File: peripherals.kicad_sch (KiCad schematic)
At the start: 36 parts, among them IC1 MIC5350-SGYMT-TR, J1 Conn_02x06_Counter_Clockwise, J2 USB_C_Receptacle_USB2.0_14P, J3 Conn_01x07, J4 Conn_01x06, J5 Conn_02x08_Odd_Even, U1 EM008LX, U2 EM008LX, U3 EM008LX, X1 2x5 0.05" SWD

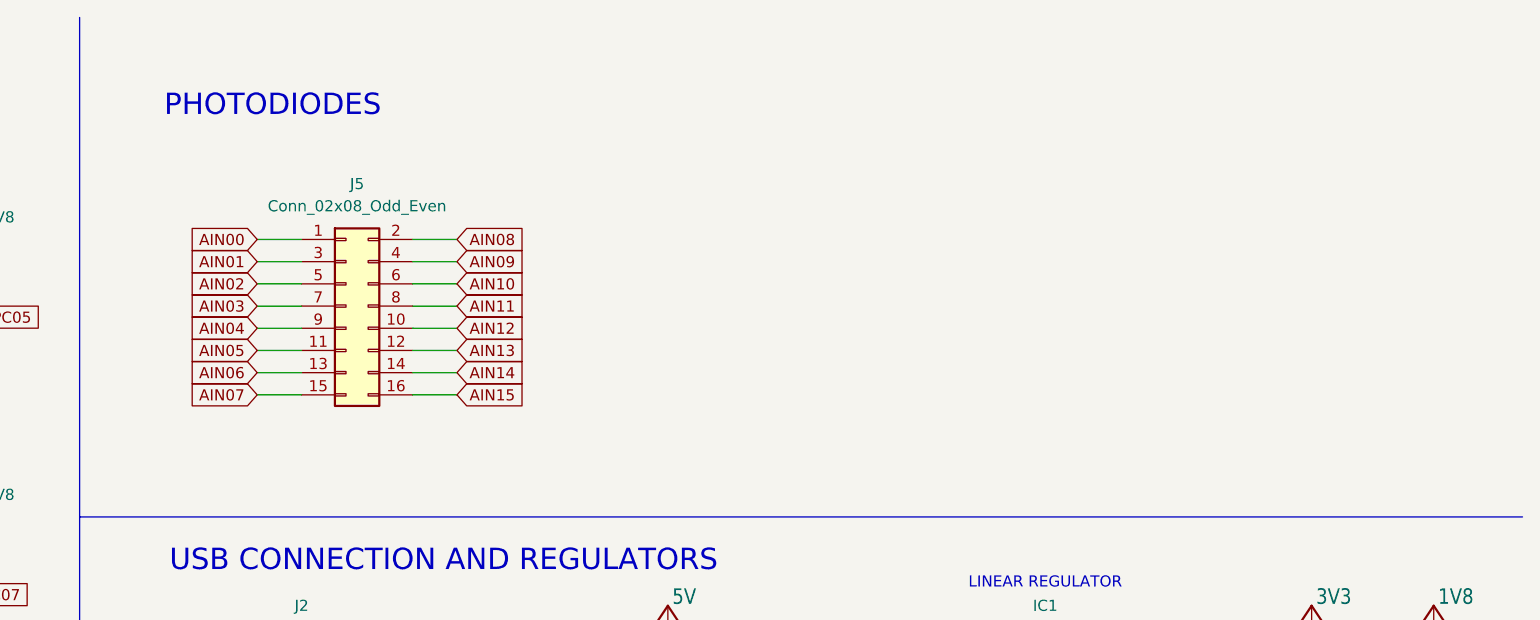
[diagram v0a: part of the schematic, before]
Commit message: Initial commit
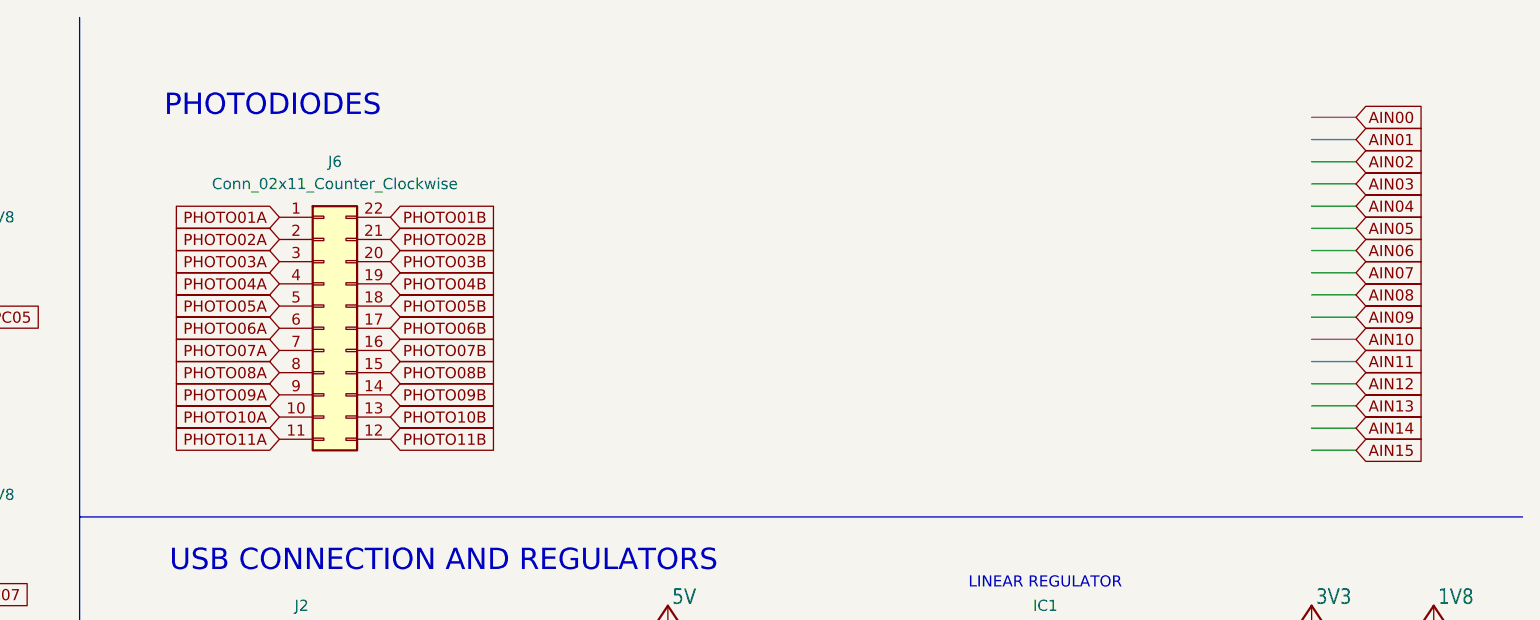
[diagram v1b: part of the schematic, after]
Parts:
- removed J5: Conn_02x08_Odd_Even, Connector_Harwin:Harwin_Gecko-G125-FVX1605L0X_2x08_P1.25mm_Vertical, symbol Connector_Generic:Conn_02x08_Odd_Even
- added J6: Conn_02x11_Counter_Clockwise, Connector_Hirose:Hirose_DF11-22DP-2DSA_2x11_P2.00mm_Vertical, symbol Connector_Generic:Conn_02x11_Counter_Clockwise
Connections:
- new net PHOTO01A: J6.1 (Pin_1)
- new net PHOTO01B: J6.22 (Pin_22)
- new net PHOTO02A: J6.2 (Pin_2)
- new net PHOTO02B: J6.21 (Pin_21)
- new net PHOTO03A: J6.3 (Pin_3)
- new net PHOTO03B: J6.20 (Pin_20)
- new net PHOTO04A: J6.4 (Pin_4)
- new net PHOTO04B: J6.19 (Pin_19)
- new net PHOTO05A: J6.5 (Pin_5)
- new net PHOTO05B: J6.18 (Pin_18)
- new net PHOTO06A: J6.6 (Pin_6)
- new net PHOTO06B: J6.17 (Pin_17)
- new net PHOTO07A: J6.7 (Pin_7)
- new net PHOTO07B: J6.16 (Pin_16)
- new net PHOTO08A: J6.8 (Pin_8)
- new net PHOTO08B: J6.15 (Pin_15)
- new net PHOTO09A: J6.9 (Pin_9)
- new net PHOTO09B: J6.14 (Pin_14)
- new net PHOTO10A: J6.10 (Pin_10)
- new net PHOTO10B: J6.13 (Pin_13)
- new net PHOTO11A: J6.11 (Pin_11)
- new net PHOTO11B: J6.12 (Pin_12)
